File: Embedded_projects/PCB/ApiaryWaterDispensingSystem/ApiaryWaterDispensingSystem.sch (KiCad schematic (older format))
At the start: 1 part

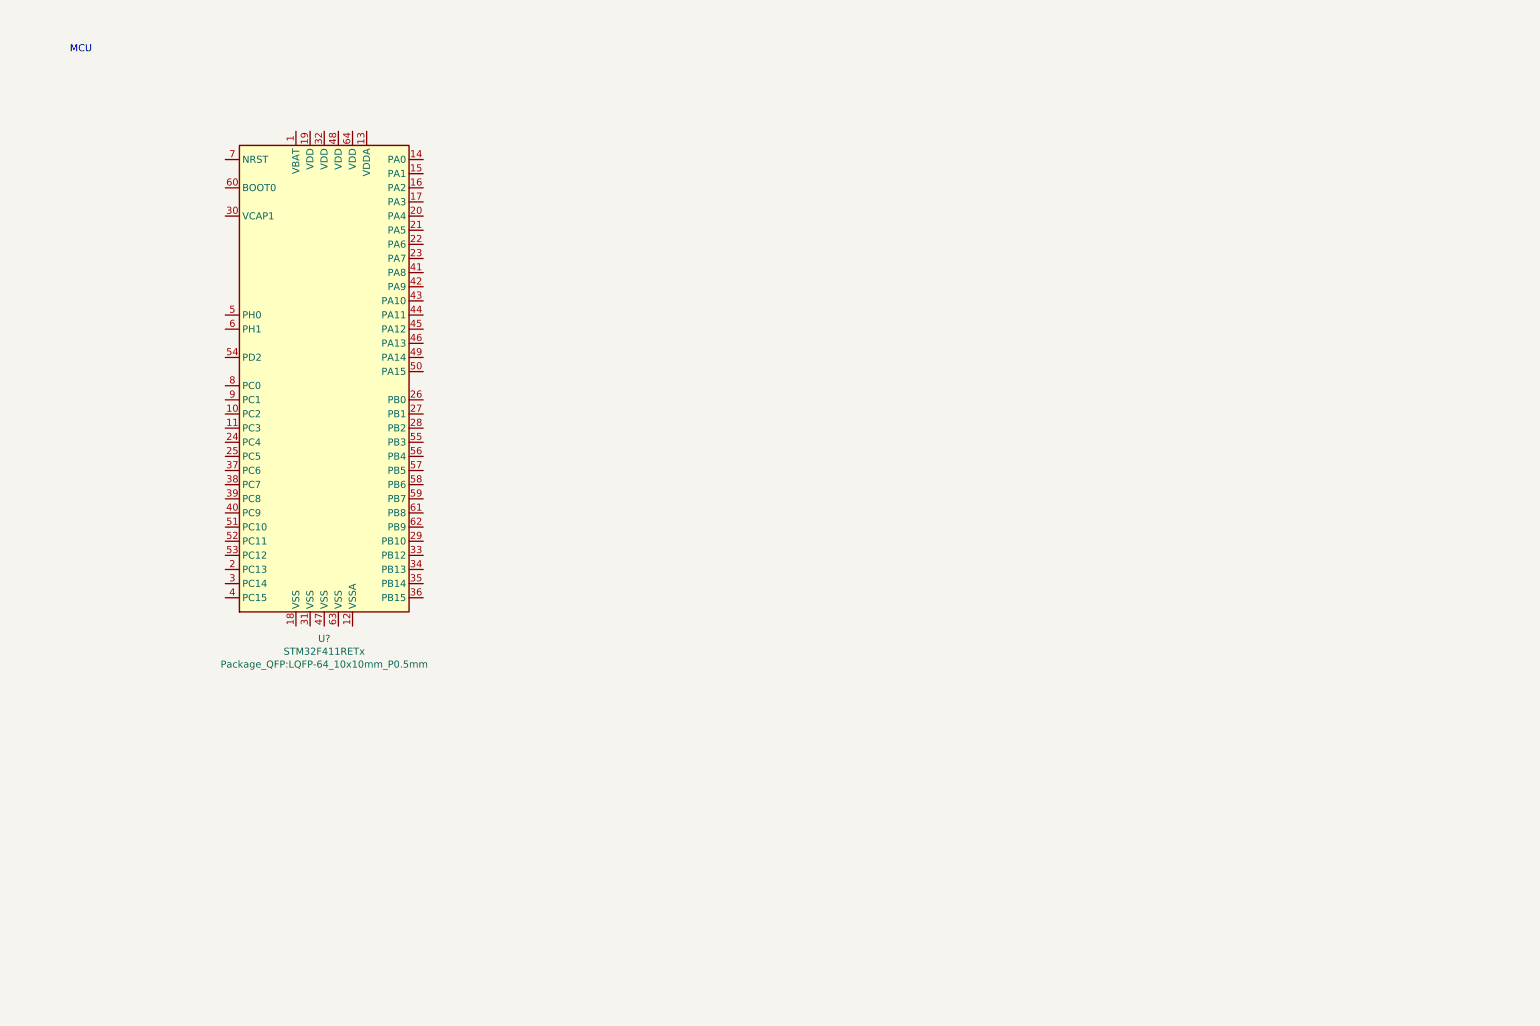
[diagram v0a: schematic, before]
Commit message: changes projects
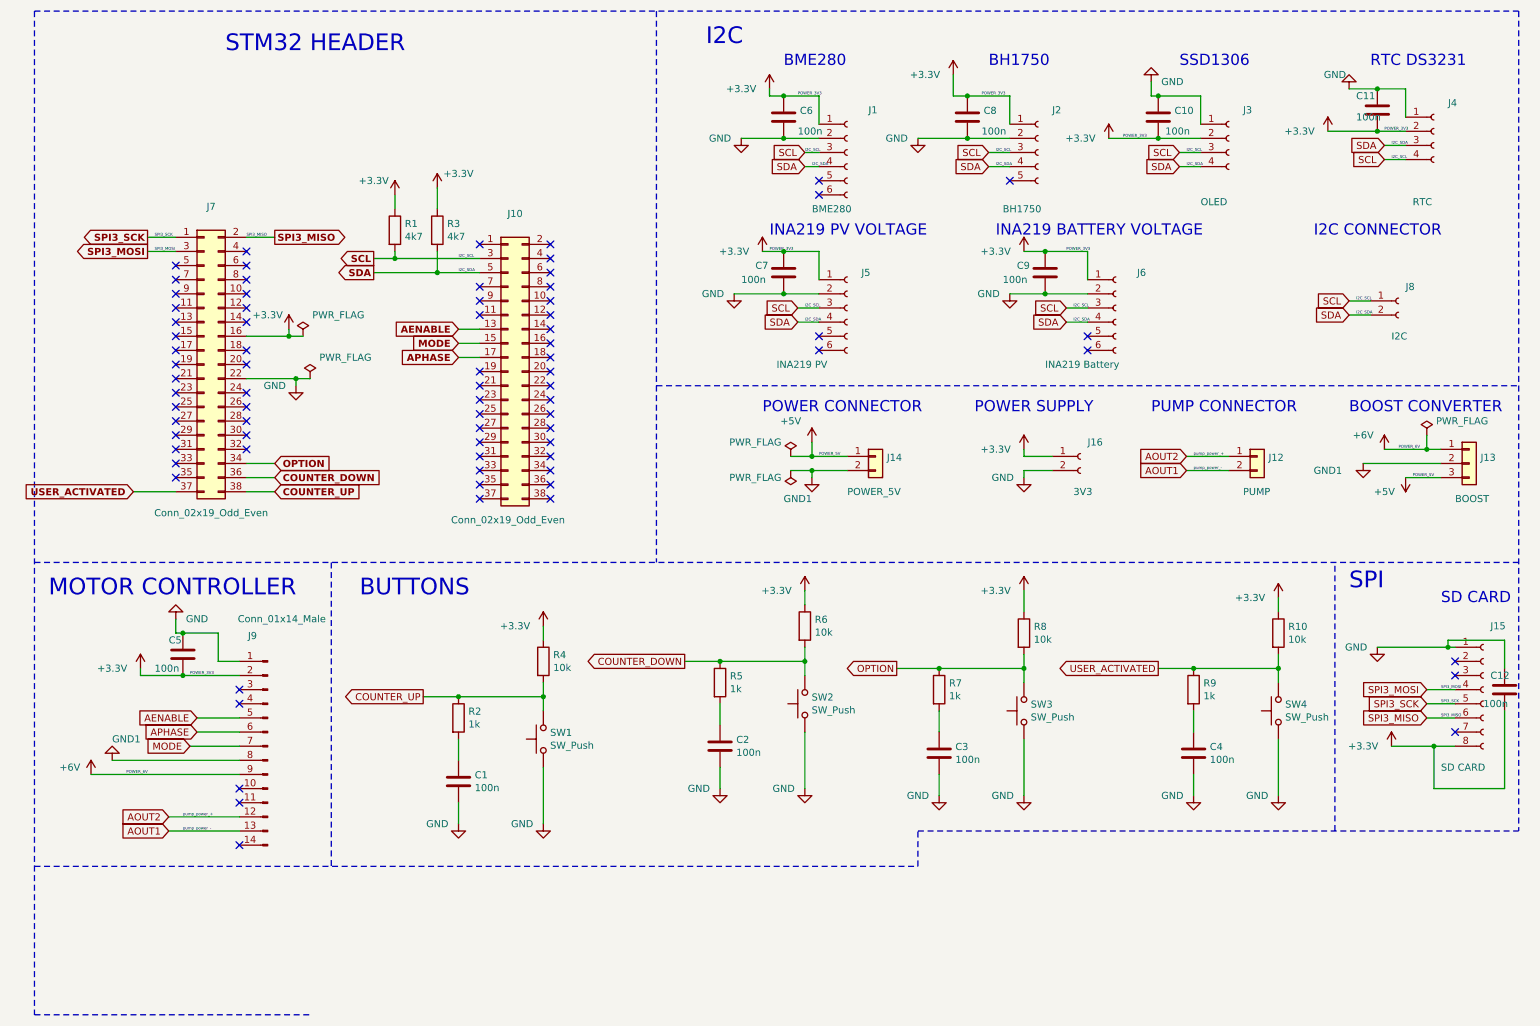
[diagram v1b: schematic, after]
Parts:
- removed U?: STM32F411RETx, Package_QFP:LQFP-64_10x10mm_P0.5mm, symbol MCU_ST_STM32F4:STM32F411RETx
- added C1, C10, C11, C12, C2, C3, C4, C5, C6, C7, C8, C9: 100n, Capacitor_SMD:C_0805_2012Metric, symbol Device:C
- added J1: BME280, ApiaryWaterDispensingSystem:PinSocket_1x06_P2.54mm_Vertical_BME280, symbol Connector:Conn_01x06_Female
- added J10, J7: Conn_02x19_Odd_Even, Connector_PinSocket_2.54mm:PinSocket_2x19_P2.54mm_Vertical, symbol Connector_Generic:Conn_02x19_Odd_Even
- added J12: PUMP, TerminalBlock_TE-Connectivity:TerminalBlock_TE_282834-2_1x02_P2.54mm_Horizontal, symbol Connector_Generic:Conn_01x02
- added J13: BOOST, Connector_PinSocket_2.00mm:PinSocket_1x03_P2.00mm_Vertical, symbol Connector_Generic:Conn_01x03
- added J14: POWER_5V, TerminalBlock_TE-Connectivity:TerminalBlock_TE_282834-2_1x02_P2.54mm_Horizontal, symbol Connector_Generic:Conn_01x02
- added J15: SD CARD, ApiaryWaterDispensingSystem:PinSocket_1x08_P2.54mm_Vertical_SD_CARD, symbol Connector:Conn_01x08_Female
- added J16: 3V3, Connector_PinSocket_2.54mm:PinSocket_1x02_P2.54mm_Vertical, symbol Connector:Conn_01x02_Female
- added J2: BH1750, Connector_PinSocket_2.54mm:PinSocket_1x05_P2.54mm_Vertical, symbol Connector:Conn_01x05_Female
- added J3: OLED, Connector_PinSocket_2.54mm:PinSocket_1x04_P2.54mm_Vertical, symbol Connector:Conn_01x04_Female
- added J4: RTC, ApiaryWaterDispensingSystem:PinSocket_1x04_P2.54mm_Vertical_RTCDS3231, symbol Connector:Conn_01x04_Female
- added J5: INA219 PV, Connector_PinSocket_2.54mm:PinSocket_1x06_P2.54mm_Vertical, symbol Connector:Conn_01x06_Female
- added J6: INA219 Battery, Connector_PinSocket_2.54mm:PinSocket_1x06_P2.54mm_Vertical, symbol Connector:Conn_01x06_Female
- added J8: I2C, Connector_PinSocket_2.54mm:PinSocket_1x02_P2.54mm_Vertical, symbol Connector:Conn_01x02_Female
- added J9: Conn_01x14_Male, ApiaryWaterDispensingSystem:PinSocket_1x07_P2.54mm_Vertical_DRV8835, symbol Connector:Conn_01x14_Male
- added R1, R3: 4k7, Resistor_SMD:R_0805_2012Metric, symbol Device:R
- added R10, R4, R6, R8: 10k, Resistor_SMD:R_0805_2012Metric, symbol Device:R
- added R2, R5, R7, R9: 1k, Resistor_SMD:R_0805_2012Metric, symbol Device:R
- added SW1, SW2, SW3, SW4: SW_Push, Button_Switch_THT:SW_PUSH-12mm, symbol Switch:SW_Push
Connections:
- new net: C1.1, R2.2
- new net: C2.1, R5.2
- new net: C3.1, R7.2
- new net: C4.1, R9.2
- new net +3V3: C10.2, C11.2, C12.2, C5.2, C6.1, C7.1, C8.1, C9.1, J1.1 (Pin_1), J15.8 (Pin_8), J16.1 (Pin_1), J2.1 (Pin_1), J3.2 (Pin_2), J4.2 (Pin_2), J5.1 (Pin_1), J6.1 (Pin_1), J7.16 (Pin_16), J9.2 (Pin_2), R1.1, R10.1, R3.1, R4.1, R6.1, R8.1
- new net +5V: J13.3 (Pin_3), J14.1 (Pin_1)
- new net +6V: J13.1 (Pin_1), J9.9 (Pin_9)
- new net AENABLE: J10.13 (Pin_13), J9.5 (Pin_5)
- new net AOUT1: J12.2 (Pin_2), J9.13 (Pin_13)
- new net AOUT2: J12.1 (Pin_1), J9.12 (Pin_12)
- new net APHASE: J10.17 (Pin_17), J9.6 (Pin_6)
- new net COUNTER_DOWN: J7.36 (Pin_36), R5.1, R6.2, SW2.2
- new net COUNTER_UP: J7.38 (Pin_38), R2.1, R4.2, SW1.2
- new net GND: C1.2, C10.1, C11.1, C12.1, C2.2, C3.2, C4.2, C5.1, C6.2, C7.2, C8.2, C9.2, J1.2 (Pin_2), J15.1 (Pin_1), J16.2 (Pin_2), J2.2 (Pin_2), J3.1 (Pin_1), J4.1 (Pin_1), J5.2 (Pin_2), J6.2 (Pin_2), J7.22 (Pin_22), J9.1 (Pin_1), SW1.1, SW2.1, SW3.1, SW4.1
- new net GND1: J13.2 (Pin_2), J14.2 (Pin_2), J9.8 (Pin_8)
- new net MODE: J10.15 (Pin_15), J9.7 (Pin_7)
- new net OPTION: J7.34 (Pin_34), R7.1, R8.2, SW3.2
- new net SCL: J1.3 (Pin_3), J10.3 (Pin_3), J2.3 (Pin_3), J3.3 (Pin_3), J4.4 (Pin_4), J5.3 (Pin_3), J6.3 (Pin_3), J8.1 (Pin_1), R1.2
- new net SDA: J1.4 (Pin_4), J10.5 (Pin_5), J2.4 (Pin_4), J3.4 (Pin_4), J4.3 (Pin_3), J5.4 (Pin_4), J6.4 (Pin_4), J8.2 (Pin_2), R3.2
- new net SPI3_MISO: J15.6 (Pin_6), J7.2 (Pin_2)
- new net SPI3_MOSI: J15.4 (Pin_4), J7.3 (Pin_3)
- new net SPI3_SCK: J15.5 (Pin_5), J7.1 (Pin_1)
- new net USER_ACTIVATED: J7.37 (Pin_37), R10.2, R9.1, SW4.2
- no-connect marks 0 -> 77
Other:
- note added: "BH1750"
- note added: "BME280"
- note added: "BOOST CONVERTER"
- note added: "BUTTONS"
- note added: "I2C CONNECTOR"
- note added: "I2C\n"
- note added: "INA219 BATTERY VOLTAGE"
- note added: "INA219 PV VOLTAGE"
- note added: "MOTOR CONTROLLER"
- note added: "POWER CONNECTOR"
- note added: "POWER SUPPLY"
- note added: "PUMP CONNECTOR"
- note added: "RTC DS3231"
- note added: "SD CARD"
- note added: "SPI"
- note added: "SSD1306"
- note added: "STM32 HEADER\n"
- note removed: "MCU"
